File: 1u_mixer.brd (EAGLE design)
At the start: 160.3 x 20 mm, 60 parts, among them IC1 TL072D, IC2 TL072D, IC3 TL072D, IC4 TL072D

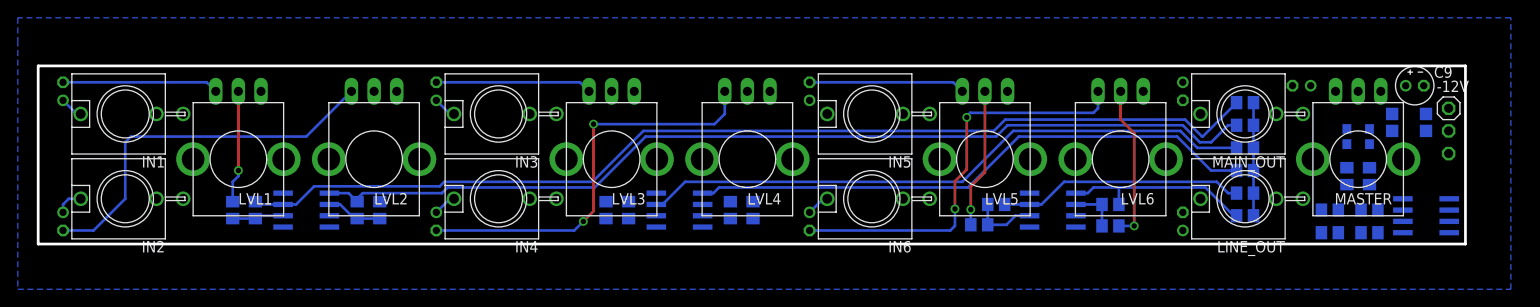
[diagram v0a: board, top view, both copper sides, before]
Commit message: asd
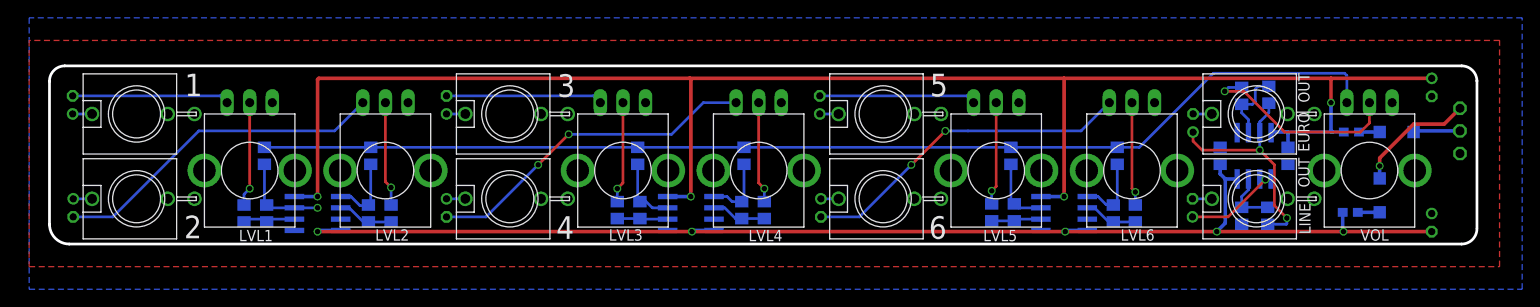
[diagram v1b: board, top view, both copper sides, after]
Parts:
- removed +12V, -12V: (no value), pinhead:1X01
- removed IN1, IN2, IN3, IN4, IN5, IN6, LINE_OUT, MAIN_OUT: WQP-PJ301M-12_JACK, thonkiconn:WQP-PJ301M-12_JACK
- removed MASTER: ALPS_POT_SMALL, jasons_stuff:SMALL_ALPS_POT
- added +12, -12: (no value), pinhead:1X01
- added 1, 2, 3, 4, 5, 6, EURO, LINE: WQP-PJ301M-12_JACK, thonkiconn:WQP-PJ301M-12_JACK
- added VOL: ALPS_POT_SMALL, jasons_stuff:SMALL_ALPS_POT
- C11, C12: device rcl:C0805 -> resistor:E2-4
- C3, C4: device resistor:E2-4 -> rcl:C0805
- moved C11 145.8 mm to (1.08, 15.6), turned to 90 degrees
- moved C12 143.0 mm to (1.14, 4.06), turned to 270 degrees
- moved C6 127.5 mm to (126.8, 4.06)
- moved R22 126.4 mm to (20.3, 3.43), turned to 270 degrees
- moved IC4 124.5 mm to (28.6, 3.43)
- moved R20 119.9 mm to (22.6, 9.91), turned to 90 degrees
- moved R21 119.4 mm to (22.9, 3.43), turned to 90 degrees
- moved C9 108.7 mm to (43.1, 15.6), flipped to the bottom, turned to 90 degrees
- moved IC1 106.6 mm to (133.7, 9.91), turned to 0 degrees
- moved R19 98.4 mm to (34.3, 3.43), turned to 90 degrees
- moved R17 98.2 mm to (34.5, 9.91), turned to 90 degrees
- moved C10 97.0 mm to (43.1, 4.06), turned to 270 degrees
- moved R18 95.9 mm to (36.8, 3.43), turned to 270 degrees
- moved C4 88.3 mm to (129.9, 9.91), turned to 270 degrees
- moved R9 87.8 mm to (106.8, 3.56), turned to 90 degrees
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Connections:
- net +12V: now also C1.+, C3.1; no longer C11.1, C9.+
- net -12V: now also C2.-, C4.2; no longer C10.-, C12.2
- net CH1: now also IC4.7, R20.1, R21.2; no longer IC1.7, R10.2, R13.1
- net CH2: now also IC4.1, R17.1, R19.2; no longer IC1.1, R12.2, R15.1
- net CH3: now also IC3.7, R14.1, R15.2; no longer IC2.7, R16.1, R6.2
- net CH4: now also IC3.1, R11.1, R13.2; no longer IC2.1, R17.1, R8.2
- net CH5: now also IC2.7, R8.1, R9.2; no longer IC3.7, R18.1, R2.2
- net CH6: now also IC2.1, R5.1, R7.2; no longer IC3.1, R19.1, R4.2
- net GND: now also 1.P$2, 1.P$3, 2.P$2, 2.P$3, 3.P$2, 3.P$3, 4.P$2, 4.P$3, 5.P$2, 5.P$3, 6.P$2, 6.P$3, C1.-, C2.+, C3.2, C4.1, EURO.P$3, IC4.3, LINE.P$3, R4.1, VOL.A; no longer C10.+, C11.2, C12.1, C9.-, IC1.3, IN1.P$2, IN1.P$3, IN2.P$2, IN2.P$3, IN3.P$2, IN3.P$3, IN4.P$2, IN4.P$3, IN5.P$2, IN5.P$3, IN6.P$2, IN6.P$3, LINE_OUT.P$3, MAIN_OUT.P$3, MASTER.A, R21.1
- net N$1: now also 5.P$1, C7.+; no longer C1.+, IN5.P$1
- net N$10: now also C9.-; no longer C4.-
- net N$11: now also IC3.6, R15.1, R16.2; no longer IC2.6, R5.2, R6.1
- net N$12: now also R16.1; no longer R5.1
- net N$13: now also 4.P$1, C10.+; no longer C5.+, IN4.P$1
- net N$14: now also C10.-; no longer C5.-
- net N$15: now also IC3.2, R12.2, R13.1; no longer IC2.2, R7.2, R8.1
- net N$16: now also R12.1; no longer R7.1
- net N$17: now also 1.P$1, C11.+; no longer C6.+, IN1.P$1
- net N$18: now also C11.-; no longer C6.-
- net N$19: now also IC4.6, R21.1, R22.2; no longer IC1.6, R10.1, R9.2
- net N$2: now also C7.-; no longer C1.-
- net N$20: now also R22.1; no longer R9.1
- net N$21: now also 2.P$1, C12.+; no longer C7.+, IN2.P$1
- net N$22: now also C12.-; no longer C7.-
- net N$23: now also IC4.2, R18.2, R19.1; no longer IC1.2, R11.2, R12.1
- net N$24: now also R18.1; no longer R11.1
- net N$25: now also R11.2, R14.2, R20.2, R5.2, R8.2, VOL.B; no longer MASTER.B, R13.2, R15.2, R16.2, R18.2, R19.2
- net N$26: now also C5.-, EURO.P$1; no longer C2.-, MAIN_OUT.P$1
- net N$27: now also C6.-, LINE.P$1; no longer C8.-, LINE_OUT.P$1
- net N$28: now also R2.1, VOL.W; no longer MASTER.W, R14.1
- net N$29: now also IC1.6, R1.1, R2.2; no longer IC4.6, R14.2, R20.1
- net N$3: now also IC2.6, R10.2, R9.1; no longer IC3.6, R1.2, R2.1
- net N$30: now also C5.+, IC1.7, R1.2, R3.1; no longer C2.+, IC4.7, R20.2, R22.1
- net N$32: now also C6.+, IC1.1, IC1.2; no longer C8.+, IC4.1, IC4.2
- net N$33: now also IC1.3, R3.2, R4.2; no longer IC4.3, R21.2, R22.2
- net N$34: now also +12.1; no longer +12V.1
- net N$36: now also -12.1; no longer -12V.1
- net N$4: now also R10.1; no longer R1.1
- net N$5: now also 6.P$1, C8.+; no longer C3.+, IN6.P$1
- net N$6: now also C8.-; no longer C3.-
- net N$7: now also IC2.2, R6.2, R7.1; no longer IC3.2, R3.2, R4.1
- net N$8: now also R6.1; no longer R3.1
- net N$9: now also 3.P$1, C9.+; no longer C4.+, IN3.P$1
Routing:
- net +12V: track 0.00 -> 188.9 mm, vias 0 -> 4
- net -12V: track 0.00 -> 144.5 mm, vias 0 -> 5
- net N$25: track 12.7 -> 128.1 mm
- net CH1: track 116.6 -> 10.5 mm, vias 0 -> 1
- net CH2: track 107.6 -> 8.24 mm
- net CH3: track 69.4 -> 7.76 mm
- net CH4: track 64.2 -> 7.65 mm
- net N$30: track 0.00 -> 26.3 mm, vias 0 -> 2
- net N$28: track 0.00 -> 22.9 mm, vias 0 -> 1
- net CH5: track 27.6 -> 7.78 mm
- net N$36: track 0.00 -> 13.6 mm, vias 0 -> 1
- net CH6: track 21.5 -> 8.08 mm
- net N$32: track 0.00 -> 11.9 mm, vias 0 -> 1
- net N$24: track 0.00 -> 11.8 mm, vias 0 -> 1
- net N$12: track 0.00 -> 11.4 mm, vias 0 -> 1
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- added copper zone on layer 1, net GND
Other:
- outline, holes or cut-outs redrawn
- board text added: "1u mini mixer v1"
- board text added: "OUT"
- board text added: "hotchk155"
